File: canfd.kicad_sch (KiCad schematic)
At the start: 12 parts

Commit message: チップ抵抗に変更
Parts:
- C? (x4): footprint Capacitor_THT:C_Disc_D4.7mm_W2.5mm_P5.00mm -> Capacitor_SMD:C_0603_1608Metric_Pad1.08x0.95mm_HandSolder
- C?: footprint Capacitor_THT:C_Disc_D4.7mm_W2.5mm_P5.00mm -> Capacitor_SMD:C_0805_2012Metric_Pad1.18x1.45mm_HandSolder
- R?: footprint Resistor_SMD:R_0201_0603Metric_Pad0.64x0.40mm_HandSolder -> Resistor_SMD:R_0805_2012Metric
- R? (x3): footprint Resistor_SMD:R_0201_0603Metric_Pad0.64x0.40mm_HandSolder -> Resistor_SMD:R_0805_2012Metric_Pad1.20x1.40mm_HandSolder
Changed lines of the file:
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@@
       (effects (font (size 1.27 1.27)) (justify right))
     )
-    (property "Footprint" "Resistor_SMD:R_0201_0603Metric_Pad0.64x0.40mm_HandSolder" (at 204.978 85.09 90)
+    (property "Footprint" "Resistor_SMD:R_0805_2012Metric" (at 204.978 85.09 90)
       (effects (font (size 1.27 1.27)) hide)
     )
@@
       (effects (font (size 1.27 1.27)))
     )
-    (property "Footprint" "Capacitor_THT:C_Disc_D4.7mm_W2.5mm_P5.00mm" (at 149.86 82.8548 0)
+    (property "Footprint" "Capacitor_SMD:C_0603_1608Metric_Pad1.08x0.95mm_HandSolder" (at 149.86 82.8548 0)
       (effects (font (size 1.27 1.27)) hide)
     )
@@
       (effects (font (size 1.27 1.27)) (justify right))
     )
-    (property "Footprint" "Capacitor_THT:C_Disc_D4.7mm_W2.5mm_P5.00mm" (at 176.8348 113.03 0)
+    (property "Footprint" "Capacitor_SMD:C_0805_2012Metric_Pad1.18x1.45mm_HandSolder" (at 176.8348 113.03 0)
       (effects (font (size 1.27 1.27)) hide)
     )
@@
       (effects (font (size 1.27 1.27)))
     )
-    (property "Footprint" "Capacitor_THT:C_Disc_D4.7mm_W2.5mm_P5.00mm" (at 149.86 108.9152 0)
+    (property "Footprint" "Capacitor_SMD:C_0603_1608Metric_Pad1.08x0.95mm_HandSolder" (at 149.86 108.9152 0)
       (effects (font (size 1.27 1.27)) hide)
     )
@@
       (effects (font (size 1.27 1.27)) (justify right))
     )
-    (property "Footprint" "Resistor_SMD:R_0201_0603Metric_Pad0.64x0.40mm_HandSolder" (at 196.088 85.09 90)
+    (property "Footprint" "Resistor_SMD:R_0805_2012Metric_Pad1.20x1.40mm_HandSolder" (at 196.088 85.09 90)
       (effects (font (size 1.27 1.27)) hide)
     )
@@
       (effects (font (size 1.27 1.27)) (justify right))
     )
-    (property "Footprint" "Resistor_SMD:R_0201_0603Metric_Pad0.64x0.40mm_HandSolder" (at 177.038 85.09 90)
+    (property "Footprint" "Resistor_SMD:R_0805_2012Metric_Pad1.20x1.40mm_HandSolder" (at 177.038 85.09 90)
       (effects (font (size 1.27 1.27)) hide)
     )
@@
       (effects (font (size 1.27 1.27)) (justify left))
     )
-    (property "Footprint" "Capacitor_THT:C_Disc_D4.7mm_W2.5mm_P5.00mm" (at 103.8352 125.73 0)
+    (property "Footprint" "Capacitor_SMD:C_0603_1608Metric_Pad1.08x0.95mm_HandSolder" (at 103.8352 125.73 0)
       (effects (font (size 1.27 1.27)) hide)
     )
@@
       (effects (font (size 1.27 1.27)))
     )
-    (property "Footprint" "Capacitor_THT:C_Disc_D4.7mm_W2.5mm_P5.00mm" (at 149.86 101.2952 0)
+    (property "Footprint" "Capacitor_SMD:C_0603_1608Metric_Pad1.08x0.95mm_HandSolder" (at 149.86 101.2952 0)
       (effects (font (size 1.27 1.27)) hide)
     )
@@
       (effects (font (size 1.27 1.27)) (justify right))
     )
-    (property "Footprint" "Resistor_SMD:R_0201_0603Metric_Pad0.64x0.40mm_HandSolder" (at 184.658 85.09 90)
-      (effects (font (size 1.27 1.27)) hide)
-    )
+    (property "Footprint" "Resistor_SMD:R_0805_2012Metric_Pad1.20x1.40mm_HandSolder" (at 184.658 85.09 90)
+      (effects (font (size 1.27 1.27)) hide)
+    )

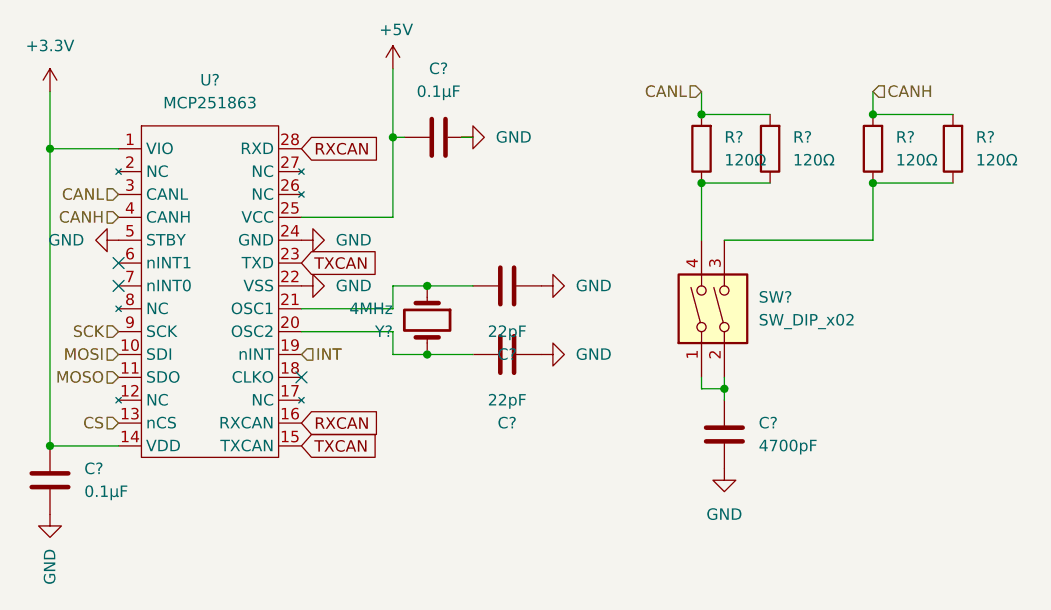
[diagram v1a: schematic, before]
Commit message: first commit
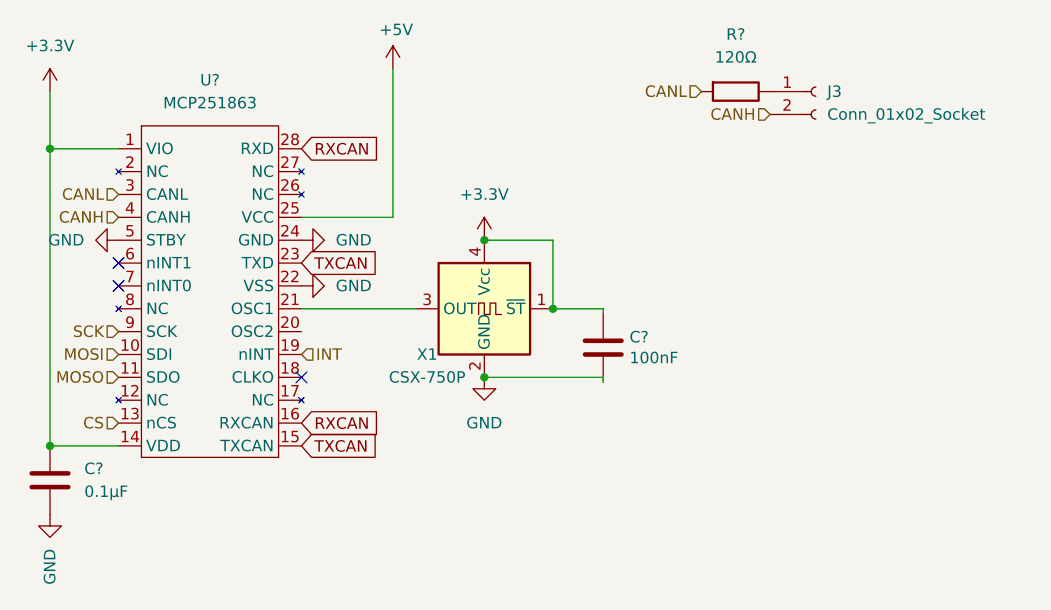
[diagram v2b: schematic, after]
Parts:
- removed C?: 0.1μF, Capacitor_SMD:C_0603_1608Metric_Pad1.08x0.95mm_HandSolder, symbol Device:C
- removed C?: 4700pF, Capacitor_SMD:C_0805_2012Metric_Pad1.18x1.45mm_HandSolder, symbol Device:C
- removed C? (x2): 22pF, Capacitor_SMD:C_0603_1608Metric_Pad1.08x0.95mm_HandSolder, symbol Device:C
- removed R?: 120Ω, Resistor_SMD:R_0805_2012Metric, symbol Device:R
- removed R? (x2): 120Ω, Resistor_SMD:R_0805_2012Metric_Pad1.20x1.40mm_HandSolder, symbol Device:R
- removed SW?: SW_DIP_x02, Button_Switch_THT:SW_DIP_SPSTx02_Slide_9.78x7.26mm_W7.62mm_P2.54mm, symbol Switch:SW_DIP_x02
- removed Y?: 4MHz, Crystal:Crystal_HC49-U_Vertical, symbol Device:Crystal
- added C?: 100nF, Capacitor_SMD:C_0805_2012Metric, symbol Device:C
- added J3: Conn_01x02_Socket, Connector_PinHeader_2.54mm:PinHeader_1x02_P2.54mm_Vertical, symbol Connector:Conn_01x02_Socket
- added X1: CSX-750P, OKL:CSX-750P, symbol oscillator:CSX-750P
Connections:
- net +3.3V: now also C?.1, X1.1 (~{ST}), X1.4 (Vcc)
- net CANH: now also J3.2 (Pin_2)
- net GND: now also C?.2, X1.2 (GND)
- net at R?.1: now also J3.1 (Pin_1)
- net at U?.21 (OSC1): now also X1.3 (OUT)
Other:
- moved on the sheet: R?
